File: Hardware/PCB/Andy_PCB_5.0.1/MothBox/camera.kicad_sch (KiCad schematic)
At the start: 8 parts

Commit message: updated footprints and schematic
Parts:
- B1: symbol MB_Library:Talentcell -> MothBox_Symbol_Library:Talentcell
- H2, H3, H4, H5, H6, H7: symbol MB_Library:MountingHole_1/4inbolt -> MothBox_Symbol_Library:MountingHole_1/4inbolt
- U19: symbol MB_Library:camera2 -> MothBox_Symbol_Library:camera2

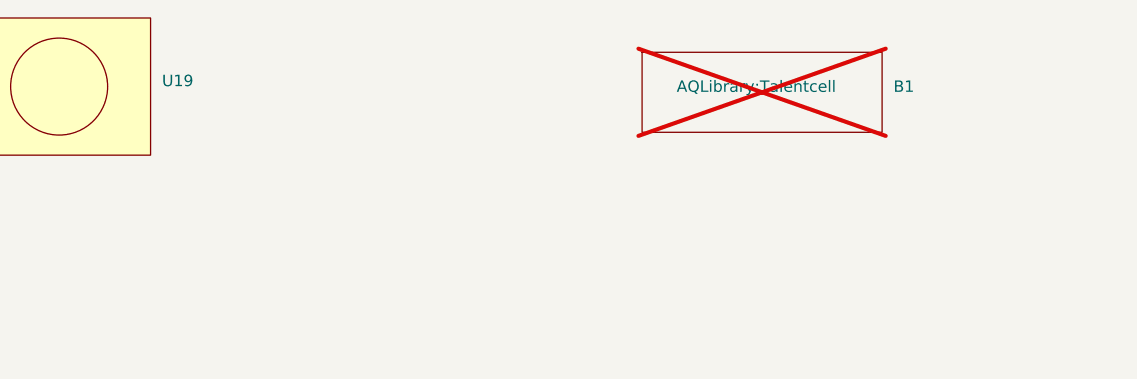
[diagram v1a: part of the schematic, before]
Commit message: daily PCB update
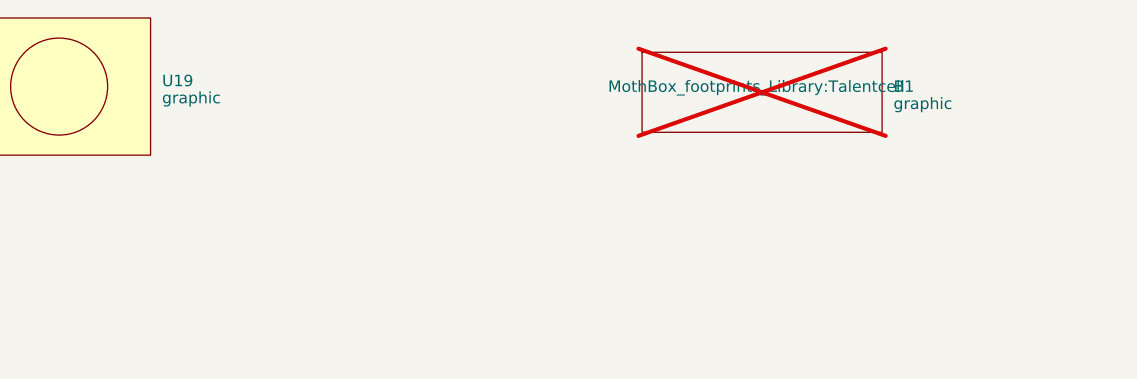
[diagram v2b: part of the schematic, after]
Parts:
- B1: value ~ -> graphic; footprint AQLibrary:Talentcell -> MothBox_footprints_Library:Talentcell
- H2, H3, H4, H5, H6, H7: footprint MountingHole:MountingHole_6.4mm_M6_Pad -> MothBox_footprints_Library:MountingHole_6.4mm_M6_Pad
- U19: value ~ -> graphic; footprint Attractor:Arducam Owlsight -> MothBox_footprints_Library:Arducam Owlsight
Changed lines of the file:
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@@
 			)
 		)
-		(property "Footprint" "MountingHole:MountingHole_6.4mm_M6_Pad"
+		(property "Footprint" "MothBox_footprints_Library:MountingHole_6.4mm_M6_Pad"
 			(at 147.32 110.49 0)
 			(effects
@@
 		)
 		(property "PRICE" ""
+			(at 147.32 110.49 0)
+			(effects
+				(font
+					(size 1.27 1.27)
+				)
+				(hide yes)
+			)
+		)
+		(property "Ali_Express_Link" ""
+			(at 147.32 110.49 0)
+			(effects
+				(font
+					(size 1.27 1.27)
+				)
+				(hide yes)
+			)
+		)
+		(property "LCSC_PN" ""
 			(at 147.32 110.49 0)
 			(effects
@@
 			)
 		)
-		(property "Footprint" "MountingHole:MountingHole_6.4mm_M6_Pad"
+		(property "Footprint" "MothBox_footprints_Library:MountingHole_6.4mm_M6_Pad"
 			(at 147.32 132.08 0)
 			(effects
@@
 		)
 		(property "PRICE" ""
+			(at 147.32 132.08 0)
+			(effects
+				(font
+					(size 1.27 1.27)
+				)
+				(hide yes)
+			)
+		)
+		(property "Ali_Express_Link" ""
+			(at 147.32 132.08 0)
+			(effects
+				(font
+					(size 1.27 1.27)
+				)
+				(hide yes)
+			)
+		)
+		(property "LCSC_PN" ""
 			(at 147.32 132.08 0)
 			(effects
@@
 			)
 		)
-		(property "Value" "~"
+		(property "Value" "graphic"
 			(at 115.57 60.96 0)
 			(effects
@@
 			)
 		)
-		(property "Footprint" "Attractor:Arducam Owlsight"
+		(property "Footprint" "MothBox_footprints_Library:Arducam Owlsight"
 			(at 104.14 59.69 0)
 			(effects
@@
 		)
 		(property "PRICE" ""
+			(at 104.14 59.69 0)
+			(effects
+				(font
+					(size 1.27 1.27)
+				)
+				(hide yes)
+			)
+		)
+		(property "Ali_Express_Link" ""
+			(at 104.14 59.69 0)
+			(effects
+				(font
+					(size 1.27 1.27)
+				)
+				(hide yes)
+			)
+		)
+		(property "LCSC_PN" ""
 			(at 104.14 59.69 0)
 			(effects
@@
 			)
 		)
-		(property "Footprint" "MountingHole:MountingHole_6.4mm_M6_Pad"
+		(property "Footprint" "MothBox_footprints_Library:MountingHole_6.4mm_M6_Pad"
 			(at 99.06 110.49 0)
 			(effects
@@
 		)
 		(property "PRICE" ""
+			(at 99.06 110.49 0)
+			(effects
+				(font
+					(size 1.27 1.27)
+				)
+				(hide yes)
+			)
+		)
+		(property "Ali_Express_Link" ""
+			(at 99.06 110.49 0)
+			(effects
+				(font
+					(size 1.27 1.27)
+				)
+				(hide yes)
+			)
+		)
+		(property "LCSC_PN" ""
 			(at 99.06 110.49 0)
 			(effects
@@
 			)
 		)
-		(property "Footprint" "MountingHole:MountingHole_6.4mm_M6_Pad"
+		(property "Footprint" "MothBox_footprints_Library:MountingHole_6.4mm_M6_Pad"
 			(at 99.06 132.08 0)
 			(effects
@@
 		)
 		(property "PRICE" ""
+			(at 99.06 132.08 0)
+			(effects
+				(font
+					(size 1.27 1.27)
+				)
+				(hide yes)
+			)
+		)
+		(property "Ali_Express_Link" ""
+			(at 99.06 132.08 0)
+			(effects
+				(font
+					(size 1.27 1.27)
+				)
+				(hide yes)
+			)
+		)
+		(property "LCSC_PN" ""
 			(at 99.06 132.08 0)
 			(effects
@@
 			)
 		)
-		(property "Footprint" "MountingHole:MountingHole_6.4mm_M6_Pad"
+		(property "Footprint" "MothBox_footprints_Library:MountingHole_6.4mm_M6_Pad"
 			(at 194.31 132.08 0)
 			(effects
@@
 		)
 		(property "PRICE" ""
+			(at 194.31 132.08 0)
+			(effects
+				(font
+					(size 1.27 1.27)
+				)
+				(hide yes)
+			)
+		)
+		(property "Ali_Express_Link" ""
+			(at 194.31 132.08 0)
+			(effects
+				(font
+					(size 1.27 1.27)
+				)
+				(hide yes)
+			)
+		)
+		(property "LCSC_PN" ""
 			(at 194.31 132.08 0)
 			(effects
@@
 			)
 		)
-		(property "Footprint" "MountingHole:MountingHole_6.4mm_M6_Pad"
+		(property "Footprint" "MothBox_footprints_Library:MountingHole_6.4mm_M6_Pad"
 			(at 194.31 110.49 0)
 			(effects
@@
 		)
 		(property "PRICE" ""
+			(at 194.31 110.49 0)
+			(effects
+				(font
+					(size 1.27 1.27)
+				)
+				(hide yes)
+			)
+		)
+		(property "Ali_Express_Link" ""
+			(at 194.31 110.49 0)
+			(effects
+				(font
+					(size 1.27 1.27)
+				)
+				(hide yes)
+			)
+		)
+		(property "LCSC_PN" ""
 			(at 194.31 110.49 0)
 			(effects
@@
 			)
 		)
-		(property "Value" "~"
+		(property "Value" "graphic"
 			(at 196.85 61.595 0)
 			(effects
@@
 			)
 		)
-		(property "Footprint" "AQLibrary:Talentcell"
+		(property "Footprint" "MothBox_footprints_Library:Talentcell"
 			(at 181.61 59.69 0)
 			(effects
@@
 			(at 181.61 59.69 0)
 			(effects
+				(font
+					(size 1.27 1.27)
+				)
+				(hide yes)
+			)
+		)
+		(property "Ali_Express_Link" ""
+			(at 181.61 59.69 0)
+			(effects
+				(font
+					(size 1.27 1.27)
+				)
+				(hide yes)
+			)
+		)
+		(property "LCSC_PN" ""
+			(at 181.61 59.69 0)
+			(effects
